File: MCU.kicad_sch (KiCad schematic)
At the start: 31 parts, among them IC1 R7FA4M1AB3CFM#AA0, J1 Conn_01x02_Pin, SW1 SW_Push, Y1 ABM8W-12.0000MHZ-8-K1Z-T3

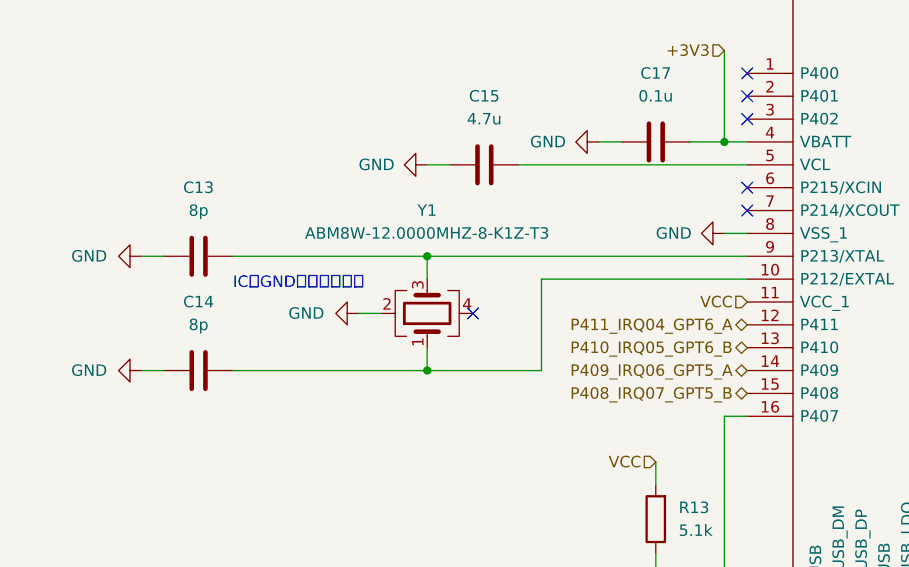
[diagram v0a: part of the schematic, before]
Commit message: 水晶振動子のGND接続方法修正
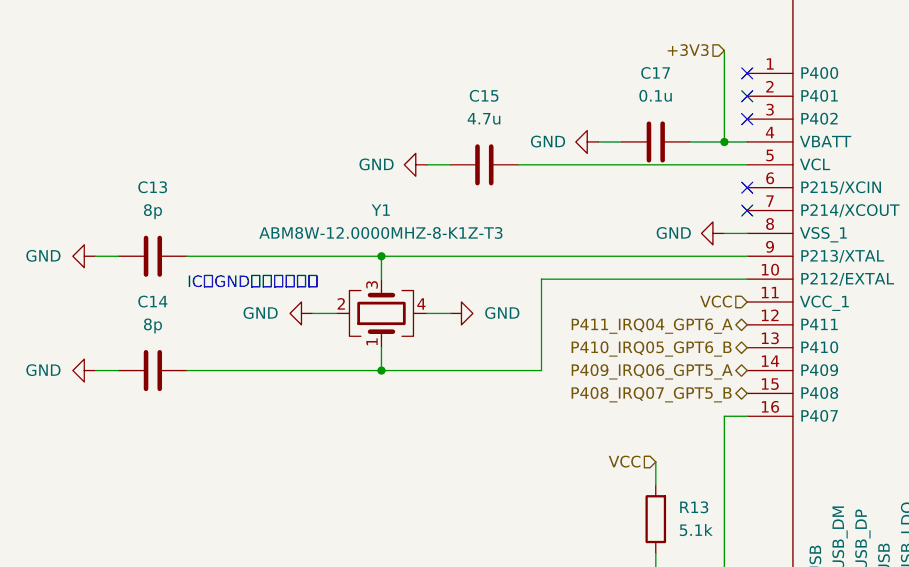
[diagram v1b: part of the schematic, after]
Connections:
- net GND: now also Y1.4
- no-connect marks 9 -> 8
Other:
- moved on the sheet: C13, C14, Y1
